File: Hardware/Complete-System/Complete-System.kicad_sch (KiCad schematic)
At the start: 1 part

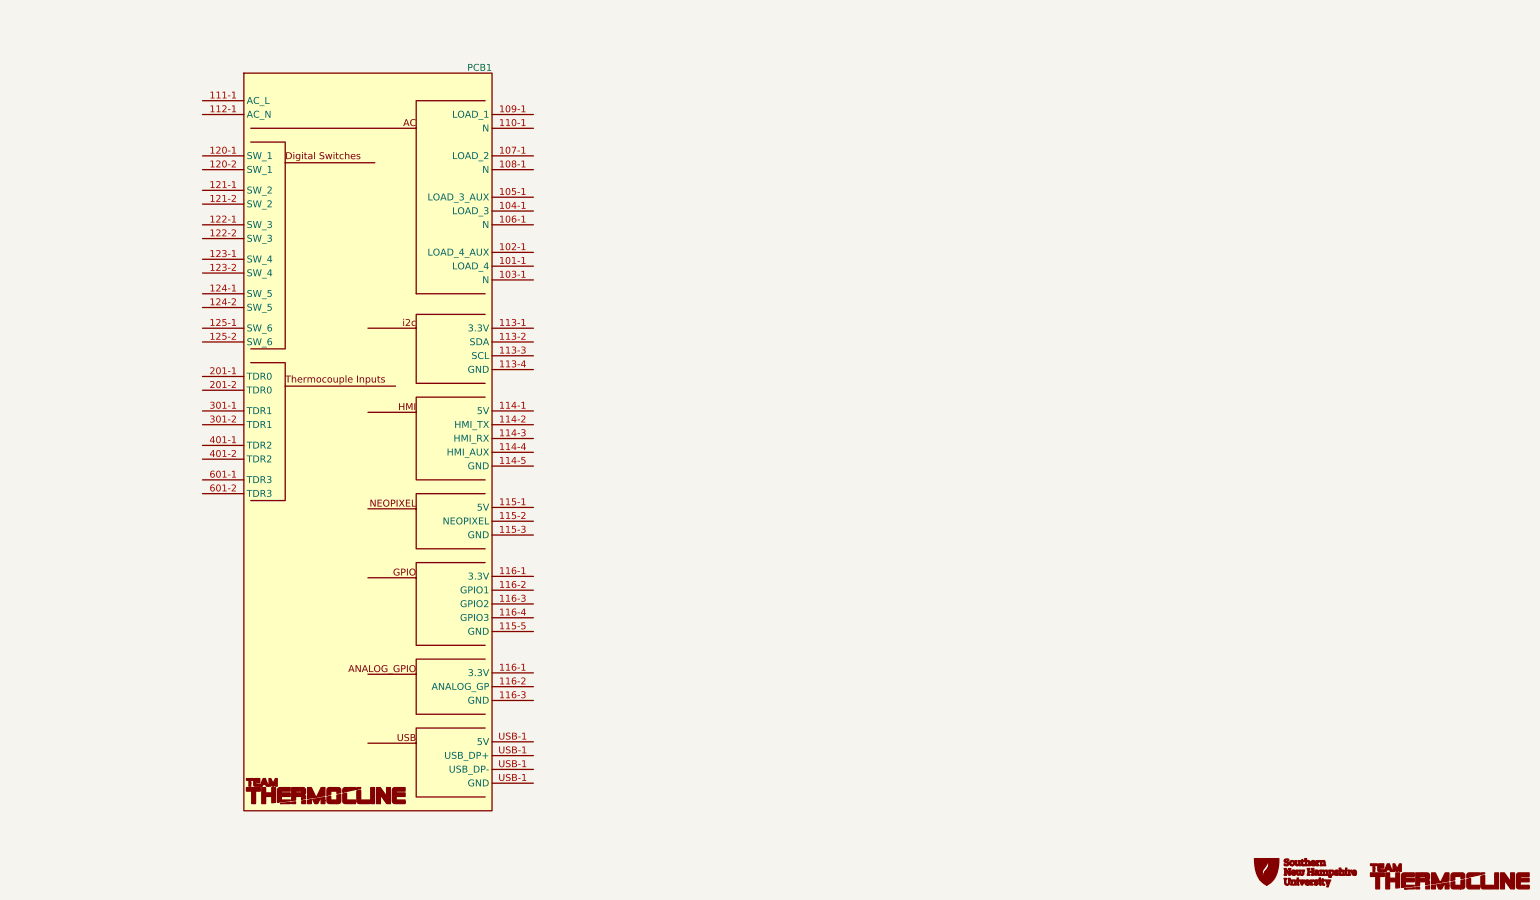
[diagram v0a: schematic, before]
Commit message: Not perfect or finished but functional for now
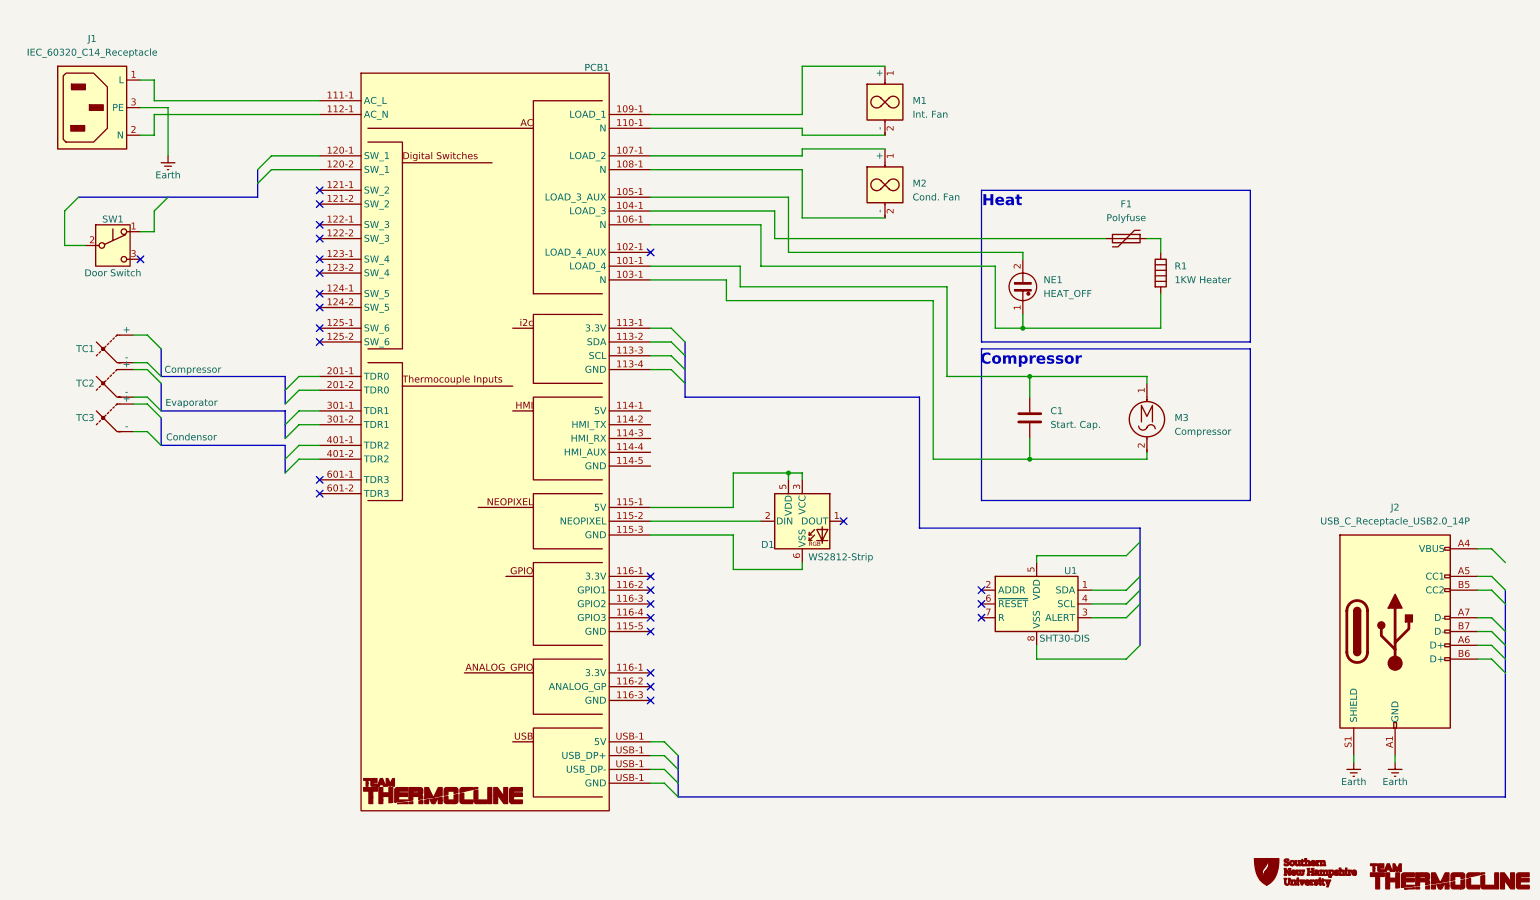
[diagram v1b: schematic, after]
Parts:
- added C1: Start. Cap., symbol Device:C
- added D1: WS2812-Strip, LED_SMD:LED_WS2812_PLCC6_5.0x5.0mm_P1.6mm, symbol LED:WS2812
- added F1: Polyfuse, symbol Device:Polyfuse
- added J1: IEC_60320_C14_Receptacle, symbol Connector:IEC_60320_C14_Receptacle
- added J2: USB_C_Receptacle_USB2.0_14P, symbol Connector:USB_C_Receptacle_USB2.0_14P
- added M1: Int. Fan, symbol Motor:Fan_IEC-60617
- added M2: Cond. Fan, symbol Motor:Fan_IEC-60617
- added M3: Compressor, symbol Motor:Motor_AC
- added NE1: HEAT_OFF, symbol Device:Lamp_Neon
- added R1: 1KW Heater, symbol Device:Heater
- added SW1: Door Switch, symbol Switch:SW_Push_SPDT
- added TC1: Compressor, symbol Device:Thermocouple
- added TC2: Evaporator, symbol Device:Thermocouple
- added TC3: Condensor, symbol Device:Thermocouple
- added U1: SHT30-DIS, Sensor_Humidity:Sensirion_DFN-8-1EP_2.5x2.5mm_P0.5mm_EP1.1x1.7mm, symbol Sensor_Humidity:SHT30-DIS
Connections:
- net at PCB1.101-1 (LOAD_4): now also C1.1, M3.1
- net at PCB1.103-1 (N): now also C1.2, M3.2
- net at PCB1.104-1 (LOAD_3): now also F1.2
- net at PCB1.105-1 (LOAD_3_AUX): now also NE1.2
- net at PCB1.106-1 (N): now also NE1.1, R1.2
- net at PCB1.107-1 (LOAD_2): now also M2.1 (+)
- net at PCB1.108-1 (N): now also M2.2 (-)
- net at PCB1.109-1 (LOAD_1): now also M1.1 (+)
- net at PCB1.110-1 (N): now also M1.2 (-)
- net at PCB1.111-1 (AC_L): now also J1.1 (L)
- net at PCB1.112-1 (AC_N): now also J1.2 (N)
- net at PCB1.115-1 (5V): now also D1.3 (VCC), D1.5 (VDD)
- net at PCB1.115-2 (NEOPIXEL): now also D1.2 (DIN)
- net at PCB1.115-3 (GND): now also D1.6 (VSS)
- new net: U1.8 (VSS), U1.9 (VSS)
- new net: F1.1, R1.1
- new net: J2.A4 (VBUS), J2.A9 (VBUS), J2.B4 (VBUS), J2.B9 (VBUS)
- new net Earth: J1.3 (PE), J2.A1 (GND), J2.A12 (GND), J2.B1 (GND), J2.B12 (GND), J2.S1 (SHIELD)
- no-connect marks 0 -> 26
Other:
- note added: "Compressor"
- note added: "Heat"
- moved on the sheet: PCB1

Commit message: More clean
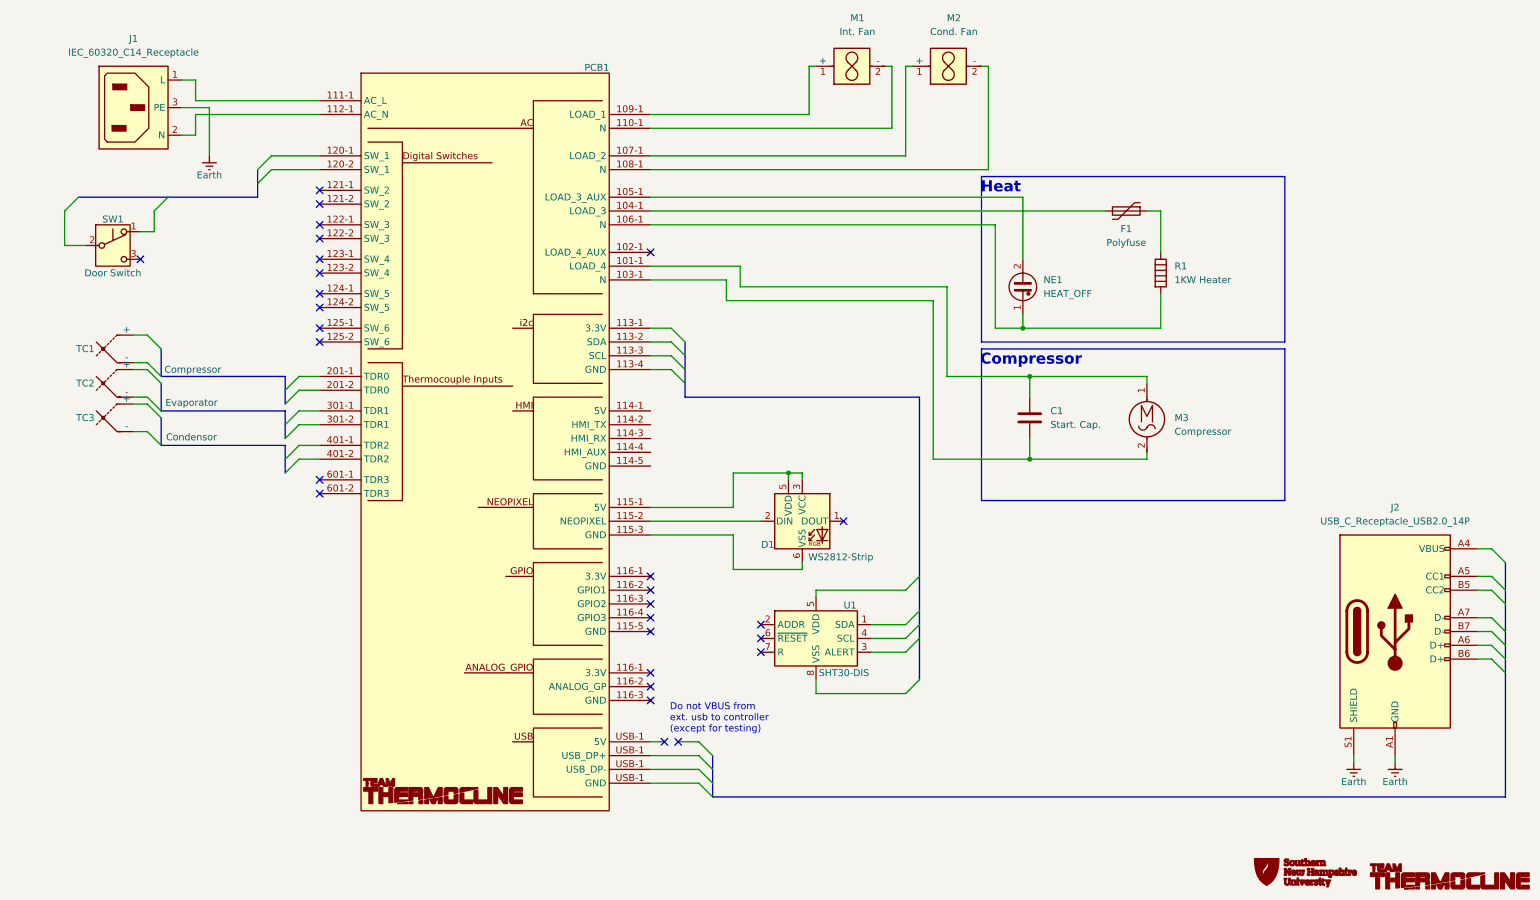
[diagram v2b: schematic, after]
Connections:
- no-connect marks 26 -> 28
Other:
- note added: "Do not VBUS from ext. usb to controller (except for testing)"
- moved on the sheet: F1, J1, M1, M2, U1
